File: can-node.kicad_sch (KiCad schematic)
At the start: 32 parts, among them J1 Conn_01x02_Pin, J2 Conn_01x02_Pin, J3 RJ45, J4 RJ45, J5 Conn_01x04_Pin, J6 Conn_01x04_Pin, J7 Screw_Terminal_01x02, SW1 SW_DIP_x04, SW2 SW_MEC_5G, SW3 SW_MEC_5G, U1 ESP32-S3, U2 MPU-9250, U3 MCP2551-I-SN

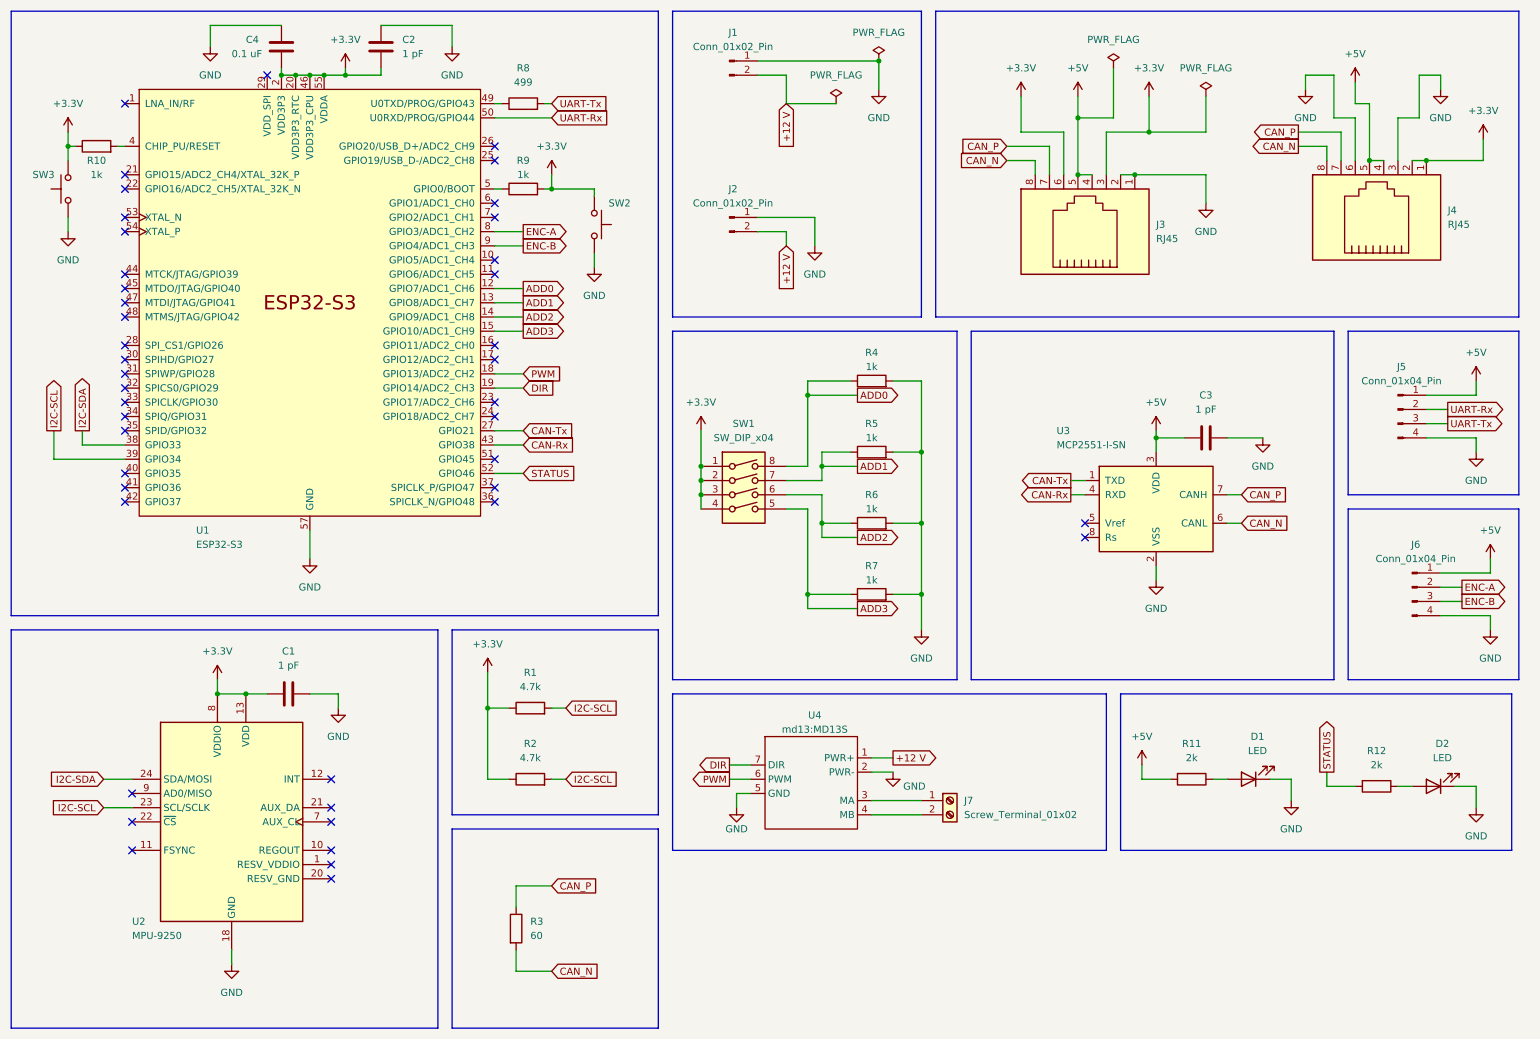
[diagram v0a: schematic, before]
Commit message: v1 for esp32 breakout
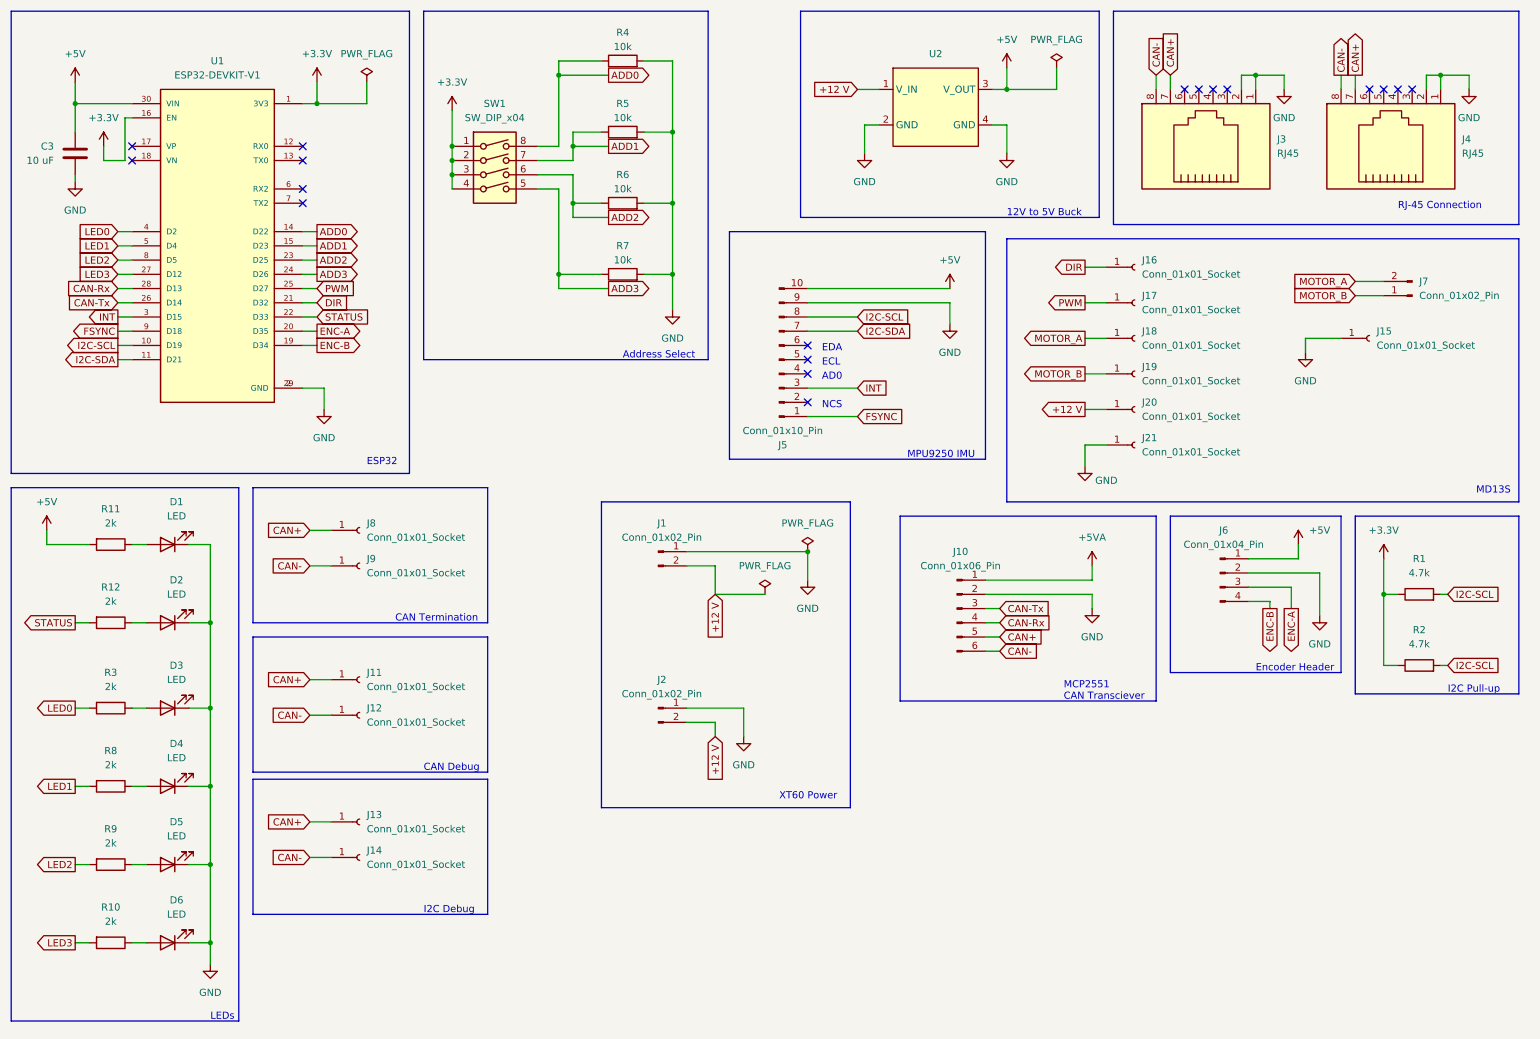
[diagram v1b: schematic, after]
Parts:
- removed C1, C2: 1 pF, Capacitor_SMD:C_0805_2012Metric_Pad1.18x1.45mm_HandSolder, symbol Device:C
- removed C4: 0.1 uF, Capacitor_SMD:C_0805_2012Metric_Pad1.18x1.45mm_HandSolder, symbol Device:C
- removed J5: Conn_01x04_Pin, Connector_PinHeader_1.00mm:PinHeader_1x04_P1.00mm_Horizontal, symbol Connector:Conn_01x04_Pin
- removed J7: Screw_Terminal_01x02, TerminalBlock:TerminalBlock_Altech_AK300-2_P5.00mm, symbol Connector:Screw_Terminal_01x02
- removed SW2, SW3: SW_MEC_5G, SMD_Buttons:SW_MEC_5GSH9, symbol Switch:SW_MEC_5G
- removed U1: ESP32-S3, Package_DFN_QFN:QFN-56-1EP_7x7mm_P0.4mm_EP5.6x5.6mm, symbol PCM_Espressif:ESP32-S3
- removed U2: MPU-9250, Sensor_Motion:InvenSense_QFN-24_3x3mm_P0.4mm, symbol Sensor_Motion:MPU-9250
- removed U3: MCP2551-I-SN, Package_SO:SOIC-8_3.9x4.9mm_P1.27mm, symbol Interface_CAN_LIN:MCP2551-I-SN
- removed U4: ~, md13:MD13S, symbol MD13S:MD13S
- added D3, D4, D5, D6: LED, LED_SMD:LED_0805_2012Metric_Pad1.15x1.40mm_HandSolder, symbol Device:LED
- added J10: Conn_01x06_Pin, Connector_PinHeader_1.00mm:PinHeader_1x06_P1.00mm_Vertical, symbol Connector:Conn_01x06_Pin
- added J11, J12, J13, J14, J8, J9: Conn_01x01_Socket, Connector_Wire:SolderWire-0.1sqmm_1x01_D0.4mm_OD1mm, symbol Connector:Conn_01x01_Socket
- added J15, J16, J17: Conn_01x01_Socket, Connector_Wire:SolderWire-0.5sqmm_1x01_D0.9mm_OD2.1mm, symbol Connector:Conn_01x01_Socket
- added J18, J19, J20, J21: Conn_01x01_Socket, Connector_Wire:SolderWire-2.5sqmm_1x01_D2.4mm_OD4.4mm, symbol Connector:Conn_01x01_Socket
- added J5: Conn_01x10_Pin, Connector_PinHeader_1.00mm:PinHeader_1x10_P1.00mm_Vertical, symbol Connector:Conn_01x10_Pin
- added J7: Conn_01x02_Pin, Connector_AMASS:AMASS_XT30U-F_1x02_P5.0mm_Vertical, symbol Connector:Conn_01x02_Pin
- added U1: ESP32-DEVKIT-V1, esp32:MODULE_ESP32_DEVKIT_V1, symbol ESP32-DEVKIT-V1:ESP32-DEVKIT-V1
- added U2: ~, MINI_360_Buck:MINI_360_Buck, symbol MINI360-buck:MINI360_Buck
- C3: value 1 pF -> 10 uF; footprint Capacitor_SMD:C_0805_2012Metric_Pad1.18x1.45mm_HandSolder -> Capacitor_SMD:C_0805_2012Metric
- R10, R9: value 1k -> 2k
- R3: value 60 -> 2k
- R4, R5, R6, R7: value 1k -> 10k
- R8: value 499 -> 2k
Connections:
- net +12 V: now also J20.1 (Pin_1), U2.1 (V_IN)
- net +3.3V: now also U1.1 (3V3), U1.16 (EN); no longer J3.3, J3.6, J4.1, J4.2, R10.1, R9.2
- net +5V: now also J5.10 (Pin_10), U1.30 (VIN), U2.3 (V_OUT); no longer J3.4, J3.5, J4.4, J4.5
- net ADD0: now also U1.14 (D22)
- net ADD1: now also U1.15 (D23)
- net ADD2: now also U1.23 (D25)
- net ADD3: now also U1.24 (D26)
- net CAN-Rx: now also J10.4 (Pin_4), U1.28 (D13)
- net CAN-Tx: now also J10.3 (Pin_3), U1.26 (D14)
- net DIR: now also J16.1 (Pin_1), U1.21 (D32)
- net ENC-A: now also J6.3 (Pin_3), U1.20 (D35); no longer J6.2 (Pin_2)
- net ENC-B: now also J6.4 (Pin_4), U1.19 (D34); no longer J6.3 (Pin_3)
- net GND: now also J4.1, J4.2, J6.2 (Pin_2), D3.1 (K), D4.1 (K), D5.1 (K), D6.1 (K), J10.2 (Pin_2), J15.1 (Pin_1), J21.1 (Pin_1), J5.9 (Pin_9), U1.2 (GND), U1.29 (GND), U2.2 (GND), U2.4 (GND); no longer J4.3, J4.6, J6.4 (Pin_4)
- net I2C-SCL: now also J5.8 (Pin_8), U1.10 (D19)
- net I2C-SDA: now also J5.7 (Pin_7), U1.11 (D21)
- net PWM: now also J17.1 (Pin_1), U1.25 (D27)
- net STATUS: now also U1.22 (D33)
- net LED3: now reaches R10.2
- net LED3: now also U1.27 (D12)
- net at R9.1: now also D5.2 (A)
- net at R8.1: now also D4.2 (A)
- net CAN_N renamed CAN-
- net CAN-: now also J10.6 (Pin_6), J12.1 (Pin_1), J14.1 (Pin_1), J9.1 (Pin_1); no longer R3.2
- net CAN_P renamed CAN+
- net CAN+: now also J10.5 (Pin_5), J11.1 (Pin_1), J13.1 (Pin_1), J8.1 (Pin_1); no longer R3.1
- net UART-Tx renamed LED1
- net LED1: now also U1.5 (D4)
- new net: D6.2 (A), R10.1
- new net: D3.2 (A), R3.1
- new net +5VA: J10.1 (Pin_1)
- new net FSYNC: J5.1 (Pin_1), U1.9 (D18)
- new net INT: J5.3 (Pin_3), U1.3 (D15)
- new net LED0: R3.2, U1.4 (D2)
- new net LED2: R9.2, U1.8 (D5)
- new net MOTOR_A: J18.1 (Pin_1), J7.2 (Pin_2)
- new net MOTOR_B: J19.1 (Pin_1), J7.1 (Pin_1)
- no-connect marks 44 -> 18
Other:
- note added: "12V to 5V Buck"
- note added: "AD0"
- note added: "Address Select"
- note added: "CAN Debug"
- note added: "CAN Termination"
- note added: "ECL"
- note added: "EDA"
- note added: "ESP32"
- note added: "Encoder Header"
- note added: "I2C Debug"
- note added: "I2C Pull-up"
- note added: "LEDs"
- note added: "MCP2551 CAN Transciever"
- note added: "MD13S"
- note added: "MPU9250 IMU"
- note added: "NCS"
- note added: "RJ-45 Connection"
- note added: "XT60 Power"
- moved on the sheet: J1, J2, J3, J4, J6, R1, R2, R4, R5, R6, R7, SW1
